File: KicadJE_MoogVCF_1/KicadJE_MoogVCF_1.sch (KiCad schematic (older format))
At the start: 0 parts

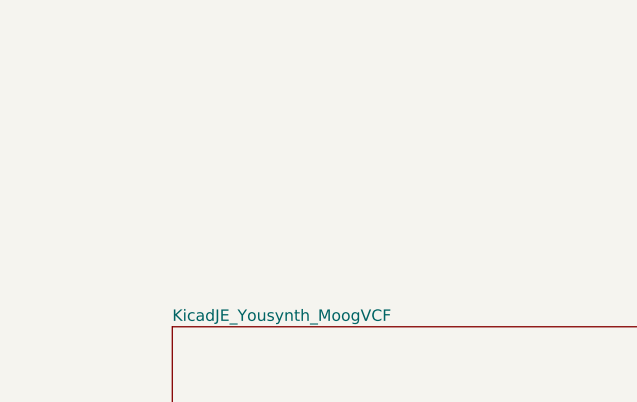
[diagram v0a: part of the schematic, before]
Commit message: acq from Ate0Ate
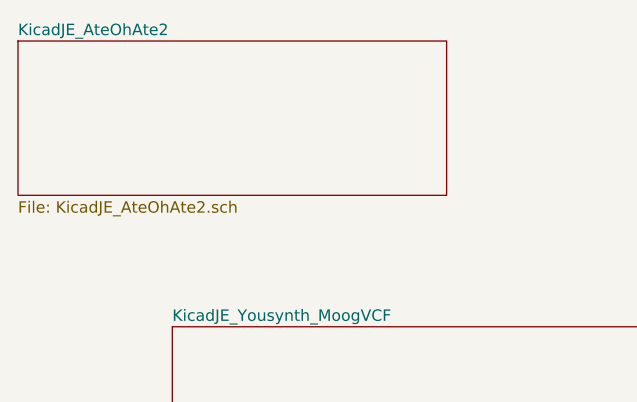
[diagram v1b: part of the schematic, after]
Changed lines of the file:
@@
 $Descr A4 11693 8268
 encoding utf-8
-Sheet 1 1
+Sheet 1 3
 Title ""
 Date ""
@@
 F1 "KicadJE_Yousynth_MoogVCF.sch" 50
 $EndSheet
+$Sheet
+S 6825 1250 1875 675
+U 5D99B81E
+F0 "KicadJE_AteOhAte2" 50
+F1 "KicadJE_AteOhAte2.sch" 50
+$EndSheet
 $EndSCHEMATC

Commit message: Footprints
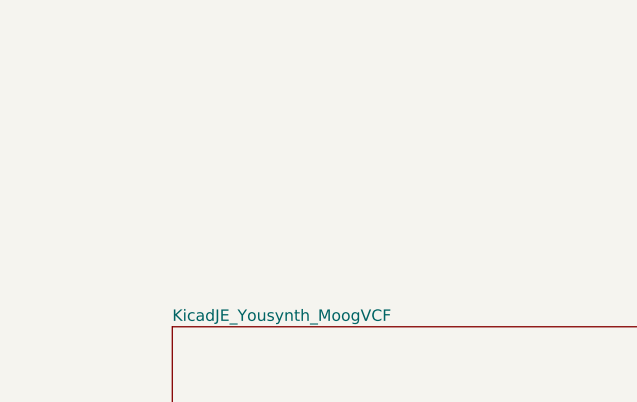
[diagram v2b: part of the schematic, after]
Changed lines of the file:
@@
 $Descr A4 11693 8268
 encoding utf-8
-Sheet 1 3
+Sheet 1 2
 Title ""
 Date ""
@@
 F1 "KicadJE_Yousynth_MoogVCF.sch" 50
 $EndSheet
-$Sheet
-S 6825 1250 1875 675
-U 5D99B81E
-F0 "KicadJE_AteOhAte2" 50
-F1 "KicadJE_AteOhAte2.sch" 50
-$EndSheet
 $EndSCHEMATC
